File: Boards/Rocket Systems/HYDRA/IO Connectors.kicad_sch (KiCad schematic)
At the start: 11 parts, among them J3 XT30UPB-F, J5 5024430270, J6 5024430570, J8 XT30UPB-F, U31 ThermoConnector, U32 ThermoConnector, U33 ThermoConnector

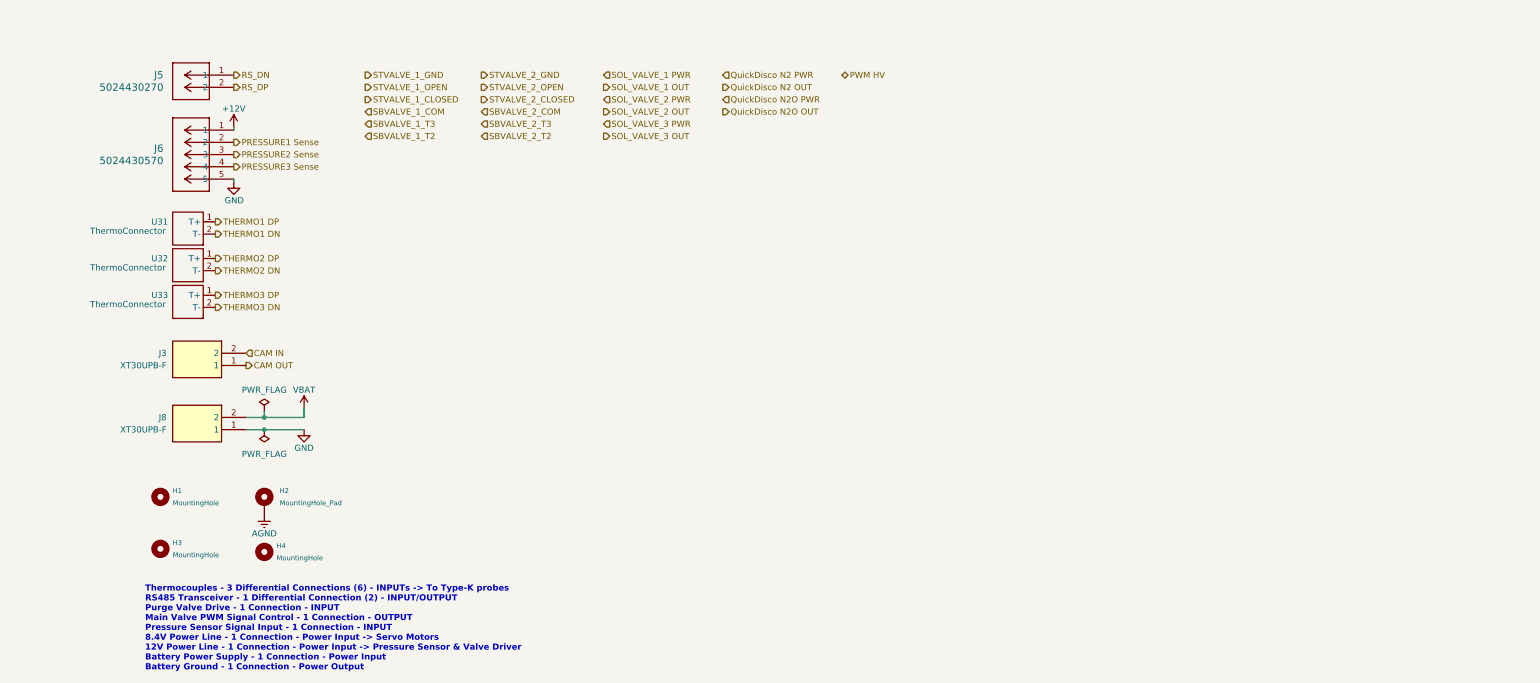
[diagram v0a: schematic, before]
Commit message: HYDRA placemenent
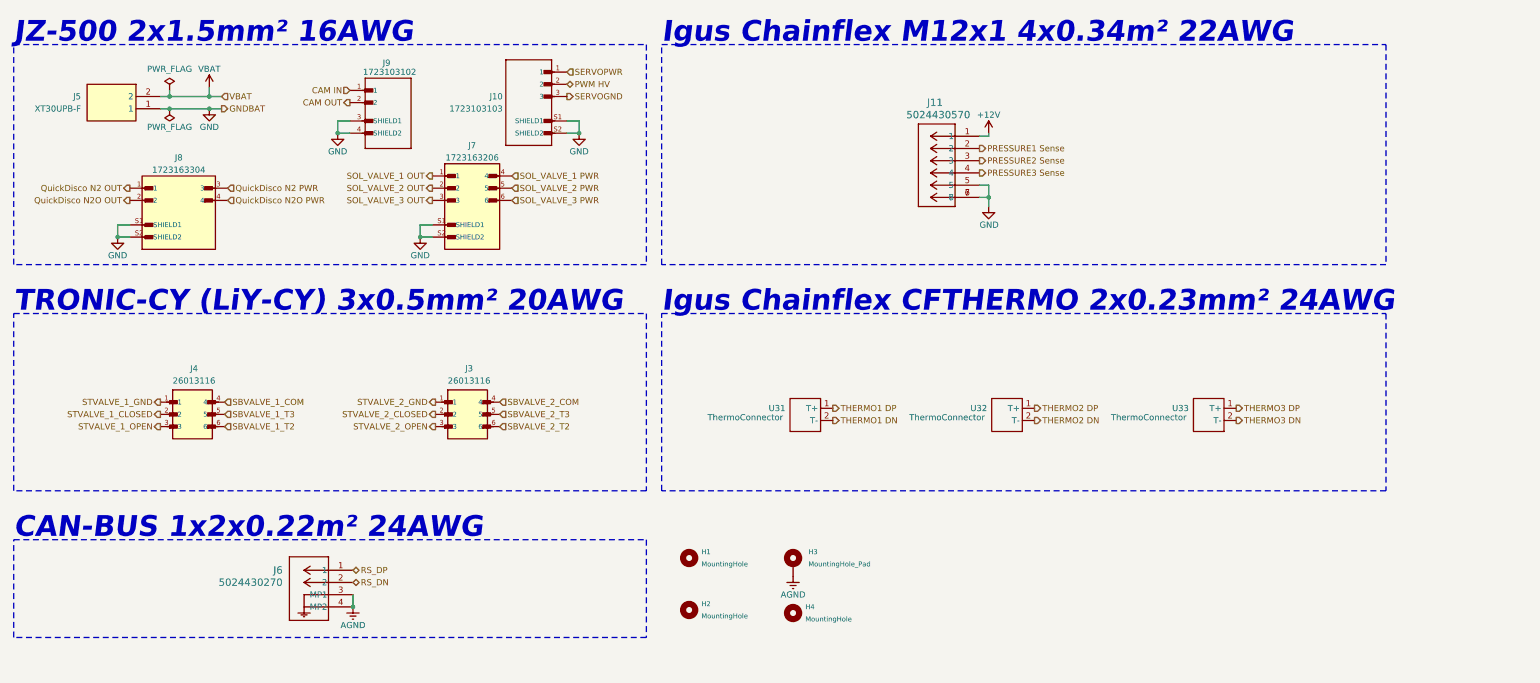
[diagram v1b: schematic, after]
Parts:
- removed J3: XT30UPB-F, XT30UPB-F:XT30UPBF, symbol XT30UPB-F:XT30UPB-F
- added J10: 1723103103, 1723103103:MOLEX_1723103103, symbol 1723103103:1723103103
- added J3, J4: 26013116, 26013116:MOLEX_26013116, symbol 26013116:26013116
- added J7: 1723163206, 1723163206:MOLEX_1723163206, symbol 1723163206:1723163206
- added J8: 1723163304, 1723163304:MOLEX_1723163304, symbol 1723163304:1723163304
- added J9: 1723103102, 1723103102:CONN02_1723103102_MOL, symbol 1723103102:1723103102
- J11: renamed from J6; footprint CONN_502443-05xx_MOL -> 5024430570:CONN_502443-05xx_MOL
- J6: renamed from J5; footprint CONN_502443-02xx_MOL -> 5024430270:CONN_502443-02xx_MOL
- renumbered H3 to H2, H2 to H3, J8 to J5
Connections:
- net AGND: now also J6.3 (MP1), J6.4 (MP2)
- net CAM IN: now also J9.1
- net CAM OUT: now also J9.2
- net GND: now also J11.6, J11.7, J10.S1 (SHIELD1), J10.S2 (SHIELD2), J7.S1 (SHIELD1), J7.S2 (SHIELD2), J8.S1 (SHIELD1), J8.S2 (SHIELD2), J9.3 (SHIELD1), J9.4 (SHIELD2)
- net PWM HV: now also J10.2
- net QuickDisco N2 OUT: now also J8.1
- net QuickDisco N2 PWR: now also J8.3
- net QuickDisco N2O OUT: now also J8.2
- net QuickDisco N2O PWR: now also J8.4
- net RS_DN: now also J6.2; no longer J6.1
- net RS_DP: now also J6.1; no longer J6.2
- net SBVALVE_1_COM: now also J4.4
- net SBVALVE_1_T2: now also J4.6
- net SBVALVE_1_T3: now also J4.5
- net SBVALVE_2_COM: now also J3.4
- net SBVALVE_2_T2: now also J3.6
- net SBVALVE_2_T3: now also J3.5
- net SOL_VALVE_1 OUT: now also J7.1
- net SOL_VALVE_1 PWR: now also J7.4
- net SOL_VALVE_2 OUT: now also J7.2
- net SOL_VALVE_2 PWR: now also J7.5
- net SOL_VALVE_3 OUT: now also J7.3
- net SOL_VALVE_3 PWR: now also J7.6
- net STVALVE_1_CLOSED: now also J4.2
- net STVALVE_1_GND: now also J4.1
- net STVALVE_1_OPEN: now also J4.3
- net STVALVE_2_CLOSED: now also J3.2
- net STVALVE_2_GND: now also J3.1
- net STVALVE_2_OPEN: now also J3.3
- new net SERVOGND: J10.3
- new net SERVOPWR: J10.1
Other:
- note added: "CAN-BUS 1x2x0.22m² 24AWG"
- note added: "Igus Chainflex CFTHERMO 2x0.23mm² 24AWG"
- note added: "Igus Chainflex M12x1 4x0.34m² 22AWG"
- note added: "JZ-500 2x1.5mm² 16AWG"
- note added: "TRONIC-CY (LiY-CY) 3x0.5mm² 20AWG"
- note removed: "Thermocouples - 3 Differential Connections (6) - INPUTs -> To Type-K probes RS485 Transceiver - 1 Differential Connection (2) - INPUT/OUTPUT Purge Valve Drive - 1 Connection - INPUT Main Valve PWM Signal Control - 1 Connection - OUTPUT Pressure Sensor Signal Input - 1 Connection - INPUT 8.4V Power Line - 1 Connection - Power Input -> Servo Motors 12V Power Line - 1 Connection - Power Input -> Pre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"
- company: (none) -> Porto Space Team
- title: (none) -> Hydraulic Regulation & Actuation system
- moved on the sheet: H1, H2, H3, H4, J5, U31, U32, U33
